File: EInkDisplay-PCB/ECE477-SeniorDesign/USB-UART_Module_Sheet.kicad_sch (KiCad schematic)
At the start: 6 parts, among them J2 USB_B, U1 CP2102-GMR

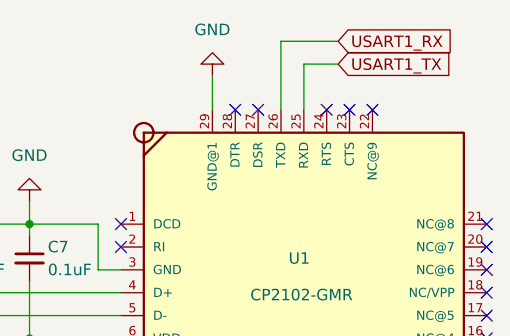
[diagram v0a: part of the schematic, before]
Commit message: push
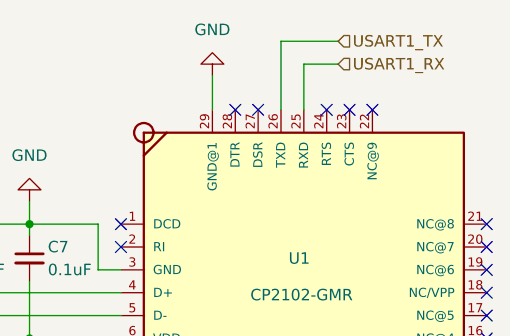
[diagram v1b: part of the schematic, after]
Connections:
- net USART1_RX: now also U1.25 (RXD); no longer U1.26 (TXD)
- net USART1_TX: now also U1.26 (TXD); no longer U1.25 (RXD)
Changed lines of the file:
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@@
-		)
-	)
-	(global_label "USART1_TX"
-		(shape input)
-		(at 167.64 69.85 0)
-		(fields_autoplaced yes)
-		(effects
-			(font
-				(size 1.27 1.27)
-			)
-			(justify left)
-		)
-		(property "Intersheetrefs" "${INTERSHEET_REFS}"
-			(at 180.8456 69.85 0)
-			(effects
-				(font
-					(size 1.27 1.27)
-				)
-				(justify left)
-				(hide yes)
-			)
-		)
-	)
-	(global_label "USART1_RX"
-		(shape input)
-		(at 167.64 67.31 0)
-		(fields_autoplaced yes)
-		(effects
-			(font
-				(size 1.27 1.27)
-			)
-			(justify left)
-		)
-		(property "Intersheetrefs" "${INTERSHEET_REFS}"
-			(at 181.148 67.31 0)
-			(effects
-				(font
-					(size 1.27 1.27)
-				)
-				(justify left)
-				(hide yes)
-			)
 		)
 	)
@@
 		)
 	)
+	(hierarchical_label "USART1_RX"
+		(shape input)
+		(at 167.64 69.85 0)
+		(effects
+			(font
+				(size 1.27 1.27)
+			)
+			(justify left)
+		)
+	)
+	(hierarchical_label "USART1_TX"
+		(shape input)
+		(at 167.64 67.31 0)
+		(effects
+			(font
+				(size 1.27 1.27)
+			)
+			(justify left)
+		)
+	)
